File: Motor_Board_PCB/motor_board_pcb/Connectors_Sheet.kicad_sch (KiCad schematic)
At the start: 14 parts, among them J10 Conn_02x03_Counter_Clockwise, J11 CSP-USC16-TR, J5 Conn_02x05_Counter_Clockwise, J8 Conn_01x02, J9 Conn_02x03_Counter_Clockwise

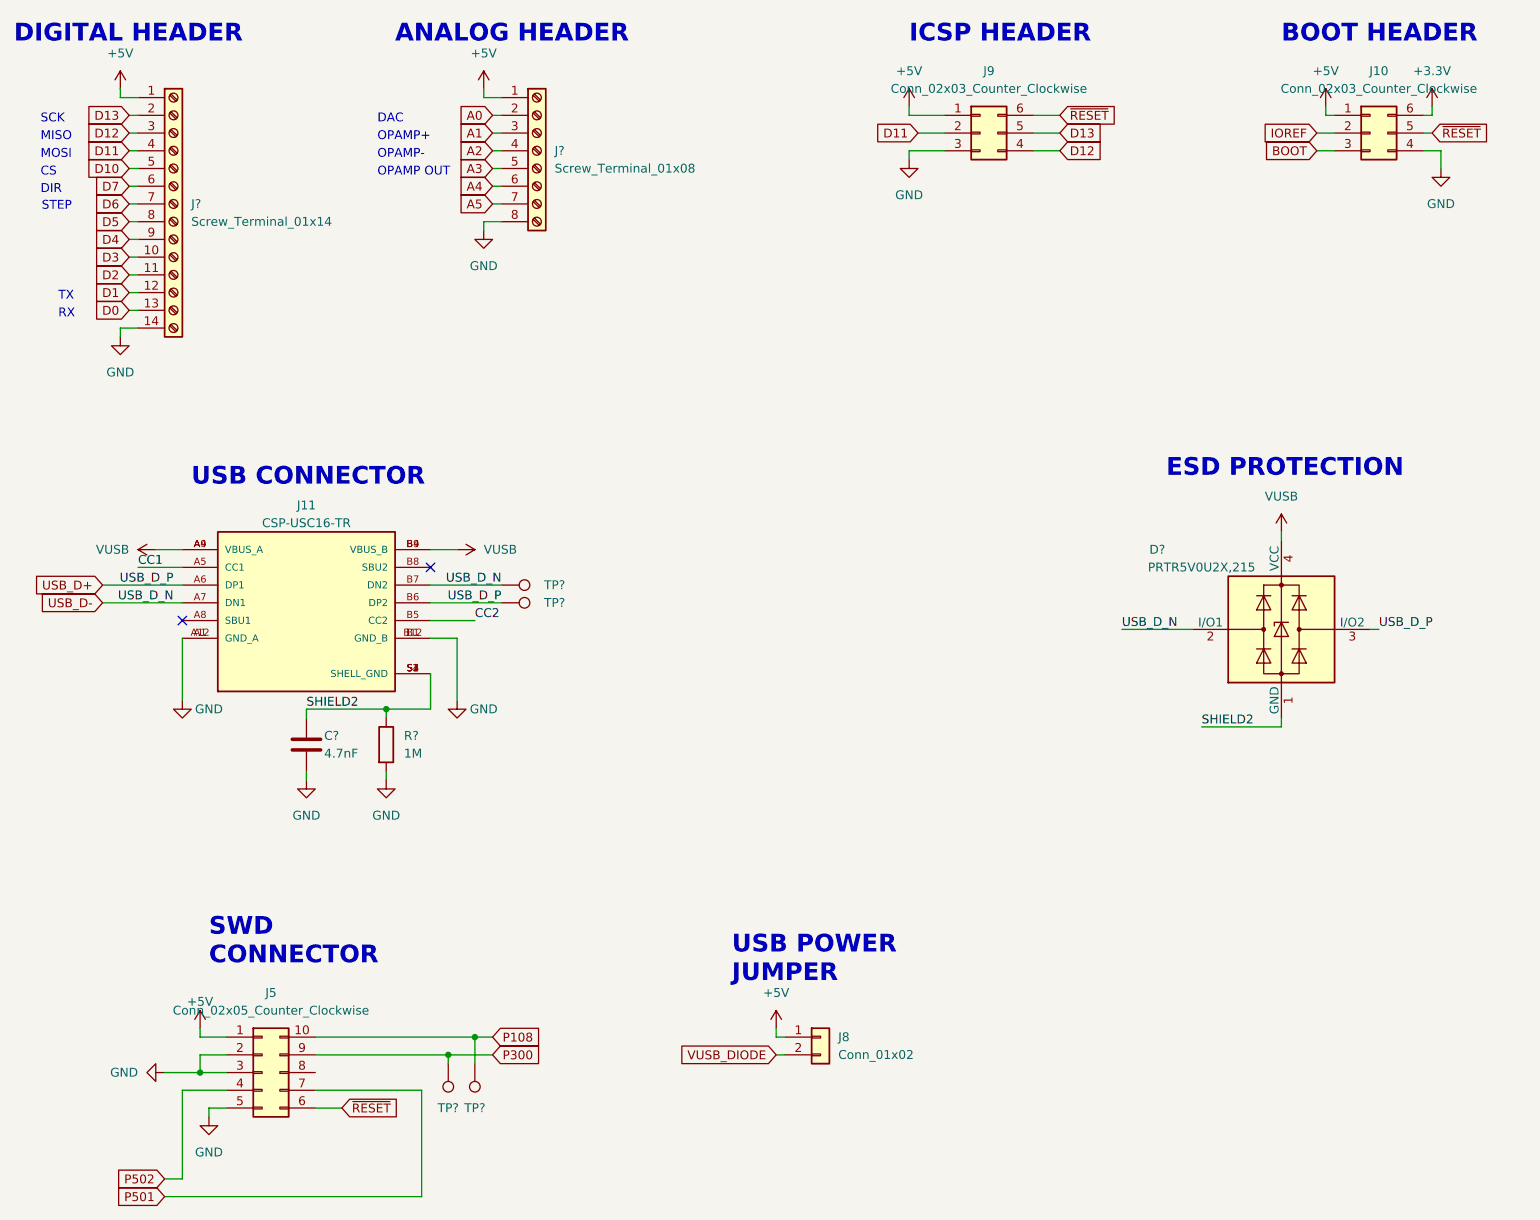
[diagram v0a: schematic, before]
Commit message: Meeting Changes
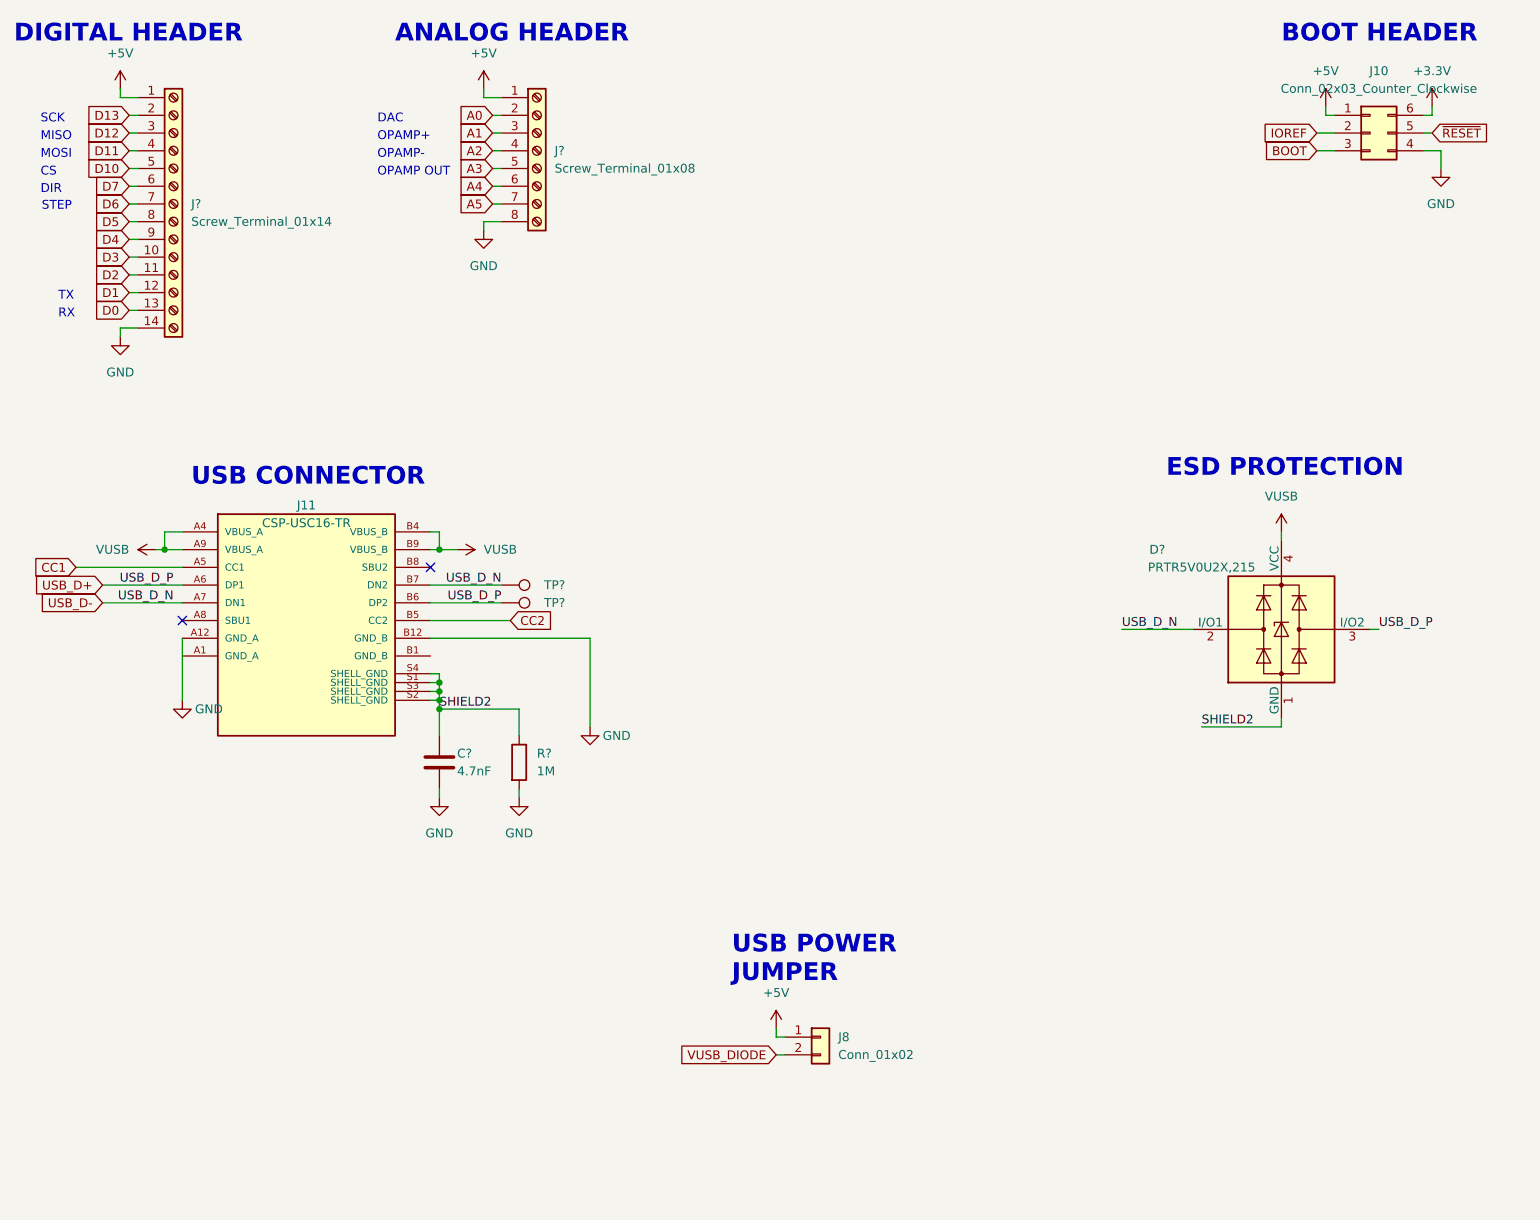
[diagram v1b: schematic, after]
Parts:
- removed J5: Conn_02x05_Counter_Clockwise, Connector_PinHeader_2.54mm:PinHeader_2x05_P2.54mm_Vertical, symbol Connector_Generic:Conn_02x05_Counter_Clockwise
- removed J9: Conn_02x03_Counter_Clockwise, Connector_PinHeader_2.54mm:PinHeader_2x03_P2.54mm_Vertical, symbol Connector_Generic:Conn_02x03_Counter_Clockwise
- removed TP? (x2): TestPoint, TestPoint:TestPoint_Pad_D1.0mm, symbol Connector:TestPoint
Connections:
- net GND: no longer J11.A1 (GND_A), J11.B1 (GND_B)
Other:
- note removed: "ICSP HEADER"
- note removed: "SWD CONNECTOR"
- moved on the sheet: C?, R?
